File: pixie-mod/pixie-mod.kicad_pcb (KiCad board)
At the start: 2 copper layers, 55 x 50 mm, 50 parts, among them J1 PWR, J2 ANT, J3 SP, J4 KEY, Q1 9018, Q2 2N3906, Q3 2N2222, Q4 2N3904, SW1 PWR, SW2 SW, U1 LM386, U2 LM78L05_TO92, U3 STC15W104, Y1 7.023MHz

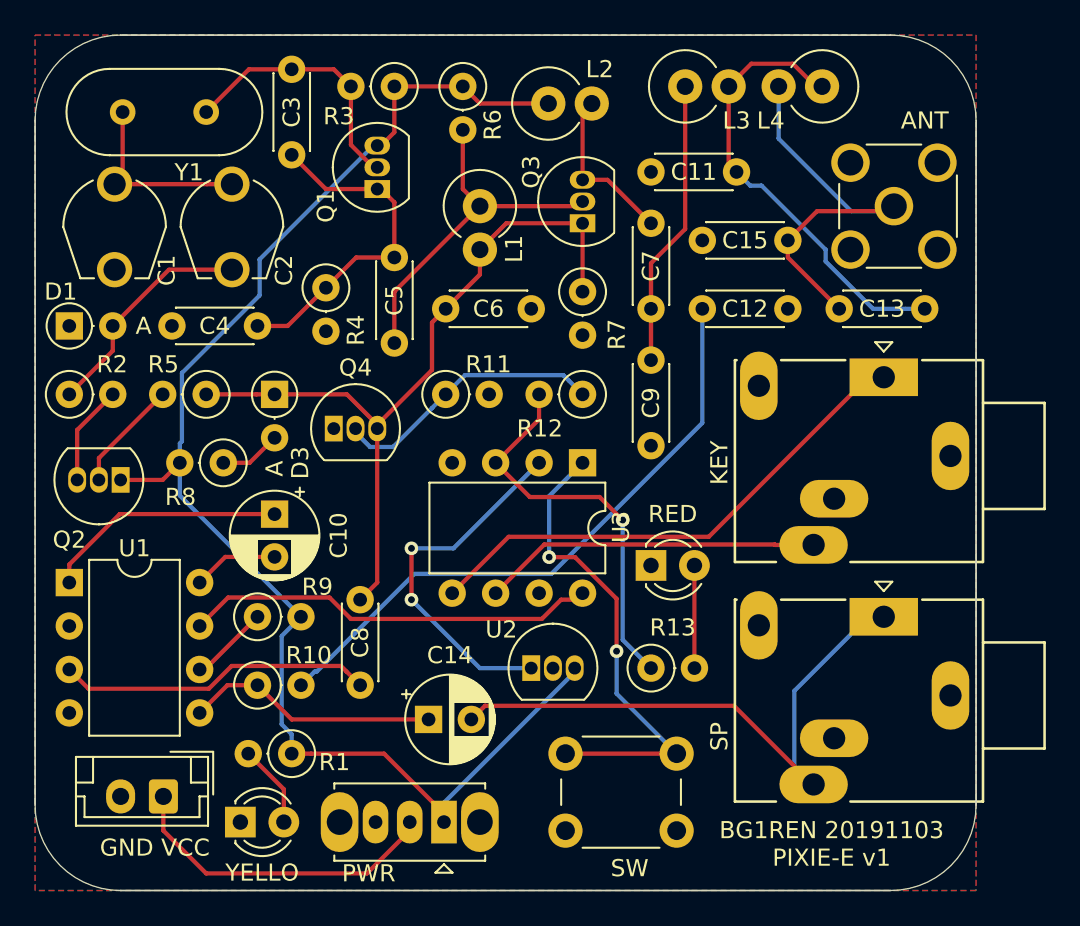
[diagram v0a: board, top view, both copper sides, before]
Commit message: Final v02
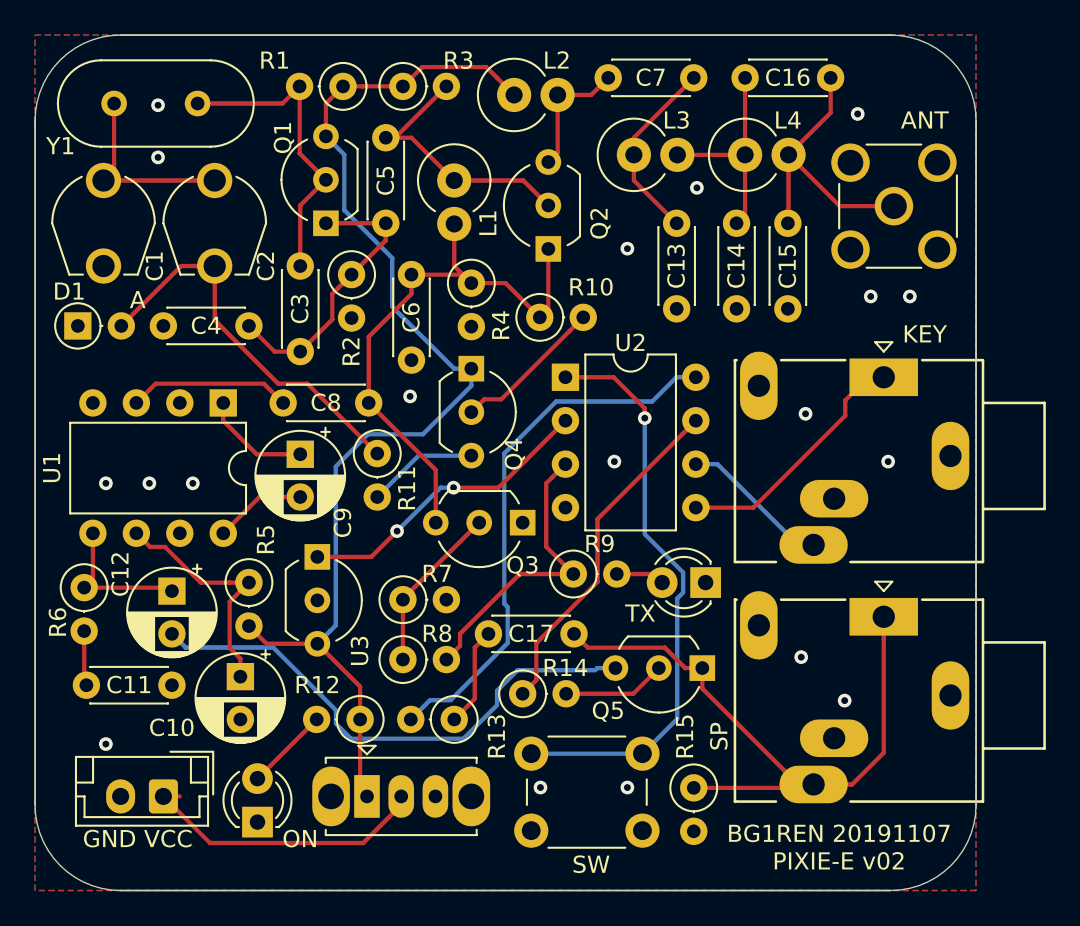
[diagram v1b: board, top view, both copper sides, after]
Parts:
- removed D4: RED, LED_THT:LED_D3.0mm
- added C16: 100, Capacitor_THT:C_Disc_D4.3mm_W1.9mm_P5.00mm, F.Cu at (146.5, 52.5)
- added C17: 100n, Capacitor_THT:C_Disc_D4.3mm_W1.9mm_P5.00mm, F.Cu at (131.5, 85.0)
- added Q5: 2N7000, Package_TO_SOT_THT:TO-92_Inline_Wide, F.Cu at (139.0, 87.0)
- added R14: 10K, Resistor_THT:R_Axial_DIN0207_L6.3mm_D2.5mm_P2.54mm_Vertical, F.Cu at (128.5, 88.5)
- added R15: 100, Resistor_THT:R_Axial_DIN0207_L6.3mm_D2.5mm_P2.54mm_Vertical, F.Cu at (138.5, 94.0)
- C1: value 50 -> 60; footprint trimmer-caps:TZ03-F -> bg1ren:TZ03-F
- C10: value 10u -> 100u
- C11: value 1n -> 10n
- C12: value 10n -> 10u; footprint Capacitor_THT:C_Disc_D4.3mm_W1.9mm_P5.00mm -> Capacitor_THT:CP_Radial_D5.0mm_P2.50mm
- C13: value 100 -> 470
- C14: value 10u -> 1n; footprint Capacitor_THT:CP_Radial_D5.0mm_P2.50mm -> Capacitor_THT:C_Disc_D4.3mm_W1.9mm_P5.00mm
- C2: value 50 -> 40; footprint trimmer-caps:TZ03-F -> bg1ren:TZ03-F
- C9: value 470 -> 10u; footprint Capacitor_THT:C_Disc_D4.3mm_W1.9mm_P5.00mm -> Capacitor_THT:CP_Radial_D5.0mm_P2.50mm
- D2: value YELLO -> RED
- D3: value 1N4148 -> YELLO; footprint Diode_THT:D_DO-35_SOD27_P2.54mm_Vertical_AnodeUp -> LED_THT:LED_D3.0mm
- Q1, Q3: footprint Package_TO_SOT_THT:TO-92_Inline -> Package_TO_SOT_THT:TO-92_Inline_Wide
- Q2: value 2N3906 -> 2N2222; footprint Package_TO_SOT_THT:TO-92_Inline -> Package_TO_SOT_THT:TO-92_Inline_Wide
- Q4: value 2N3904 -> 2N3906; footprint Package_TO_SOT_THT:TO-92_Inline -> Package_TO_SOT_THT:TO-92_Inline_Wide
- R1: value 4.7K -> 47K
- R10: value 10 -> 4.7K
- R11, R13: value 2K -> 4.7K
- R12: value 1K -> 4.7K
- R2: value 4.7K -> 470
- R4: value 470 -> 10K
- R5: value 4.7K -> 1K
- R6: value 47K -> 10
- R7: value 10K -> 2K
- R9: value 1K -> 2K
- U2: value LM78L05_TO92 -> STC15W104; footprint Package_TO_SOT_THT:TO-92_Inline -> Package_DIP:DIP-8_W7.62mm
- U3: value STC15W104 -> LM78L05_TO92; footprint Package_DIP:DIP-8_W7.62mm -> Package_TO_SOT_THT:TO-92_Inline_Wide
- moved C11 41.0 mm to (108.0, 88.0), turned to 180 degrees
- moved C12 39.6 mm to (108.0, 82.5), turned to 270 degrees
- moved R1 39.1 mm to (118.0, 53.0)
- moved R6 36.7 mm to (102.9, 82.3)
- moved D2 30.6 mm to (139.2, 82.0), turned to 180 degrees
- moved C14 30.0 mm to (141.0, 66.0), turned to 90 degrees
- moved Q2 28.4 mm to (130.0, 62.5), turned to 90 degrees
- moved R10 27.1 mm to (129.5, 66.5)
- moved D3 25.0 mm to (113.0, 96.0), turned to 90 degrees
- moved R12 23.0 mm to (119.0, 90.0)
- moved R7 20.8 mm to (121.5, 83.0), turned to 0 degrees
- moved C9 20.5 mm to (115.5, 74.5), turned to 270 degrees
- moved R9 18.6 mm to (131.5, 81.5)
- moved R2 17.9 mm to (118.5, 64.0), turned to 270 degrees
- moved Q3 17.8 mm to (128.5, 78.5), turned to 180 degrees
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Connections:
- C10 pad 1: Net-(C10-Pad1) -> /V+
- C10 pad 2: Net-(C10-Pad2) -> GND
- C12 pad 1: GND -> Net-(C12-Pad1)
- C12 pad 2: Net-(C12-Pad2) -> AF
- C13 pad 1: ANT -> GND
- C13 pad 2: Net-(C11-Pad2) -> LPF
- C14 pad 1: Net-(C14-Pad1) -> GND
- C14 pad 2: Phone -> Net-(C14-Pad2)
- C2 pad 2: Net-(C2-Pad2) -> SHIFT
- C8 pad 1: Net-(C8-Pad1) -> KEY
- C8 pad 2: KEY -> Net-(C8-Pad2)
- C9 pad 1: GND -> Net-(C9-Pad1)
- C9 pad 2: LPF -> Net-(C9-Pad2)
- D1 pad 2: Net-(C2-Pad2) -> SHIFT
- D3 pad 1: KEY -> GND
- L3 pad 2: Net-(C11-Pad2) -> Net-(C14-Pad2)
- L4 pad 1: Net-(C11-Pad2) -> Net-(C14-Pad2)
- Q2 pad 1: VCC -> KEY
- Q2 pad 2: Net-(Q2-Pad2) -> Net-(C5-Pad1)
- Q2 pad 3: Net-(Q2-Pad3) -> Net-(C7-Pad2)
- Q3 pad 1: KEY -> GND
- Q3 pad 2: Net-(C5-Pad1) -> Net-(Q3-Pad2)
- Q3 pad 3: Net-(C7-Pad2) -> KEY
- Q4 pad 1: GND -> VCC
- Q4 pad 3: KEY -> Net-(Q4-Pad3)
- R1 pad 2: Net-(D2-Pad2) -> Net-(C3-Pad1)
- R10 pad 1: Net-(C14-Pad1) -> KEY
- R10 pad 2: Net-(C12-Pad2) -> Net-(Q4-Pad2)
- R11 pad 1: Net-(Q4-Pad2) -> SHIFT
- R11 pad 2: GND -> Net-(Q4-Pad3)
- R12 pad 1: Net-(Q4-Pad2) -> VCC
- R12 pad 2: Net-(R12-Pad2) -> Net-(D3-Pad2)
- R13 pad 1: Net-(R12-Pad2) -> Net-(C17-Pad2)
- R13 pad 2: Net-(D4-Pad2) -> Sidetone
- R2 pad 1: Net-(C2-Pad2) -> Net-(C3-Pad2)
- R2 pad 2: Net-(Q2-Pad3) -> GND
- R3 pad 2: Net-(C3-Pad1) -> Net-(C5-Pad1)
- R4 pad 1: Net-(C3-Pad2) -> KEY
- R5 pad 1: KEY -> /V+
- R5 pad 2: Net-(Q2-Pad2) -> VCC
- R6 pad 1: VCC -> Net-(C12-Pad1)
- R6 pad 2: Net-(C5-Pad1) -> Net-(C11-Pad2)
- R7 pad 1: KEY -> Net-(Q3-Pad2)
- R8 pad 1: Net-(D3-Pad2) -> Net-(Q3-Pad2)
- R8 pad 2: VCC -> Net-(R8-Pad2)
- R9 pad 1: Net-(R9-Pad1) -> Net-(R8-Pad2)
- R9 pad 2: VCC -> Net-(D2-Pad2)
- U1 pad 1: Net-(C10-Pad1) -> Net-(C9-Pad1)
- U1 pad 3: Net-(C8-Pad1) -> Net-(C8-Pad2)
- U1 pad 5: Net-(C14-Pad1) -> Net-(C12-Pad1)
- U1 pad 6: Net-(R9-Pad1) -> /V+
- U1 pad 7: Sidetone -> (no net)
- U1 pad 8: Net-(C10-Pad2) -> Net-(C9-Pad2)
- U2 pad 1: 5V -> SW
- U2 pad 2: GND -> 5V
- U2 pad 3: VCC -> Net-(R8-Pad2)
- U3 pad 1: SW -> 5V
- U3 pad 2: 5V -> GND
- U3 pad 3: Net-(R12-Pad2) -> VCC
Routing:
- net Net-(C12-Pad2): track 36.5 -> 0.00 mm
- net AF: track 0.00 -> 31.1 mm
- net Net-(R12-Pad2): track 23.2 -> 0.00 mm, vias 1 -> 0
- net Net-(C11-Pad2): track 26.0 -> 3.22 mm
- net SHIFT: track 0.00 -> 22.8 mm
- net MUTE: track 0.00 -> 20.2 mm
- net Net-(C8-Pad1): track 18.5 -> 0.00 mm
- net Net-(R8-Pad2): track 0.00 -> 17.4 mm
- net VCC: track 84.4 -> 68.4 mm
- net DIT: track 30.5 -> 14.7 mm
- net Net-(C14-Pad1): track 14.9 -> 0.00 mm
- net Net-(C10-Pad1): track 14.3 -> 0.00 mm
- net /V+: track 0.00 -> 14.0 mm
- net Net-(C2-Pad2): track 13.4 -> 0.00 mm
- net Net-(C14-Pad2): track 0.00 -> 12.7 mm
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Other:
- board text added: "BG1REN 20191107 PIXIE-E v02"
- board text removed: "BG1REN 20191103 PIXIE-E v1"
